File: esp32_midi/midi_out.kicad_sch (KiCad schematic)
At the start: 3 parts, among them J6 MIDI 1 OUT, Q4 BSS138

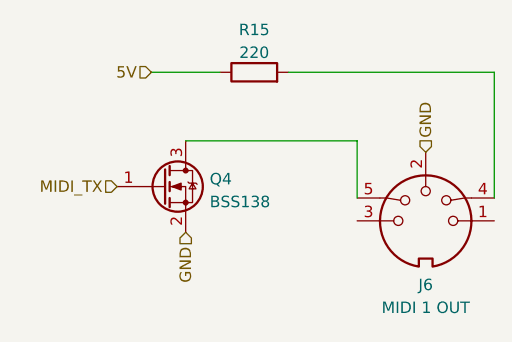
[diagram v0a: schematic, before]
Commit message: Started work on PCB
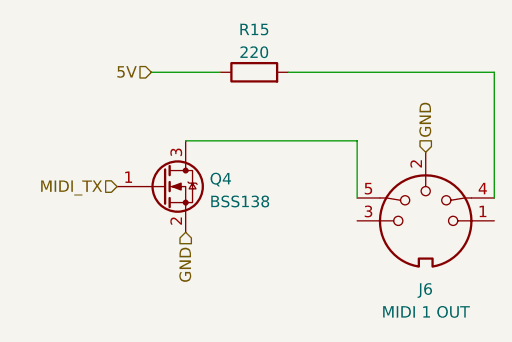
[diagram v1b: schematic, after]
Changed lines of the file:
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@@
   (symbol (lib_id "Connector:DIN-5_180degree") (at 114.3 67.31 0) (mirror y) (unit 1)
     (in_bom yes) (on_board yes) (dnp no) (fields_autoplaced)
-    (property "Reference" "J6" (at 114.2999 74.4204 0)
+    (property "Reference" "J6" (at 114.2999 74.93 0)
       (effects (font (size 1.27 1.27)))
     )
-    (property "Value" "MIDI 1 OUT" (at 114.2999 76.9573 0)
+    (property "Value" "MIDI 1 OUT" (at 114.2999 77.47 0)
       (effects (font (size 1.27 1.27)))
     )
